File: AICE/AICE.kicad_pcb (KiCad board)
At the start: 2 copper layers, 90 x 85 mm, 140 parts, among them J1 Conn_02x10_Odd_Even, J2 Conn_02x10_Odd_Even, J3 Conn_01x03, J4 USB_A, J5 Conn_02x10_Odd_Even, J6 Conn_02x10_Odd_Even, J8 USB_B_Micro, Q1 S8550, U1 ICE40UP5K-SG48ITR, U11 DVP_PORT, U12 SMS, U13 ZLDO1117G33TA, U14 XC6206P122MR, U15 ZLDO1117G33TA, U16 ZLDO1117G18TA, U17 XC6206P282MR, U18 XC6206P152MR, U2 ASFLMB-24.00MHZ-LC-T, U3 SMS, U4 W25Q, U5 HX711, U6 Omega2+, U7 SMS, U8 SRF2012, U9 M1&M1W

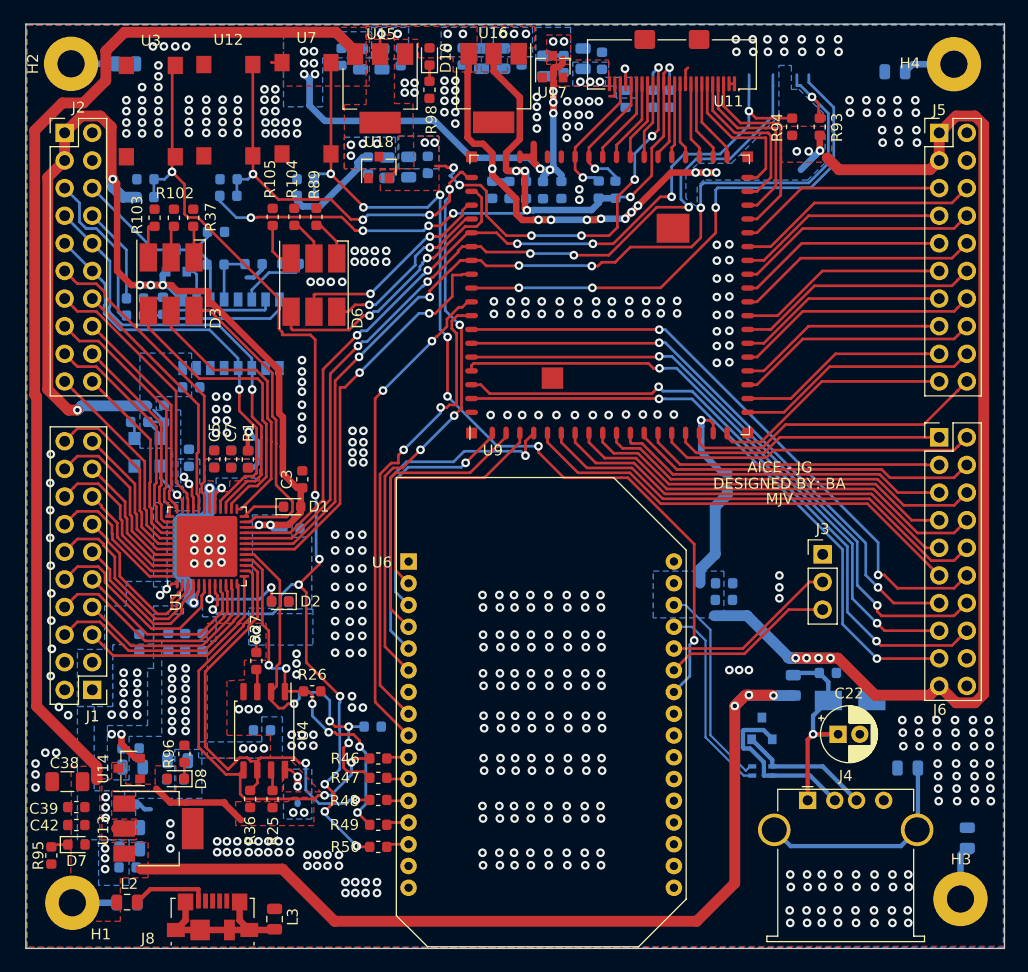
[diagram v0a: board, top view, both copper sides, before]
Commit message: Add files via upload
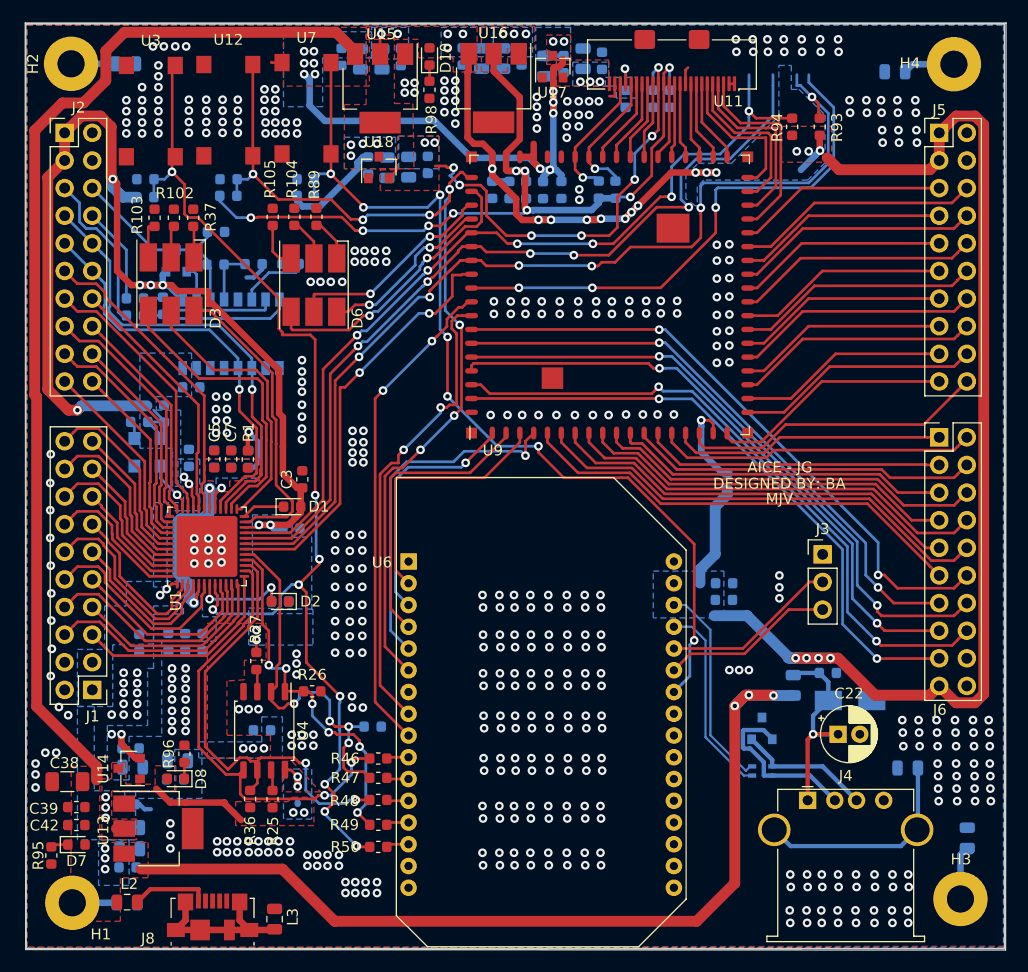
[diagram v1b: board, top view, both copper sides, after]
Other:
- board size 90 x 85 mm -> 90.2 x 85.2 mm
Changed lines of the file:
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@@
   (general
     (thickness 1.6)
-    (drawings 10)
+    (drawings 14)
     (tracks 2330)
     (zones 0)
@@
     )
   )
+  (gr_line (start 123.15 63.9) (end 123.1 149.15) (layer Edge.Cuts) (width 0.1))
+  (gr_line (start 32.95 63.9) (end 123.15 63.9) (layer Edge.Cuts) (width 0.1))
+  (gr_line (start 33 149.1) (end 32.95 63.9) (layer Edge.Cuts) (width 0.1))
+  (gr_line (start 123.1 149.15) (end 33 149.1) (layer Edge.Cuts) (width 0.1))
+  (gr_line (start 123 148.998) (end 33.006 148.998) (layer Edge.Cuts) (width 0.05))
+  (gr_line (start 33.006 148.998) (end 33.006 63.998) (layer Edge.Cuts) (width 0.05))
+  (gr_line (start 33.006 63.998) (end 123 63.998) (layer Edge.Cuts) (width 0.05))
+  (gr_line (start 123 63.998) (end 123 143) (layer Edge.Cuts) (width 0.05))
   (gr_text MJV (at 102.3 107.65) (layer F.SilkS)
     (effects (font (size 1 1) (thickness 0.25)))
@@
     (effects (font (size 1 1) (thickness 0.15) italic))
   )
-  (gr_line (start 123 148.998) (end 33.006 148.998) (layer Edge.Cuts) (width 0.05))
   (gr_line (start 123 143) (end 123 149) (layer Edge.Cuts) (width 0.05))
-  (gr_line (start 123 63.998) (end 123 143) (layer Edge.Cuts) (width 0.05))
-  (gr_line (start 33.006 63.998) (end 123 63.998) (layer Edge.Cuts) (width 0.05))
-  (gr_line (start 33.006 148.998) (end 33.006 63.998) (layer Edge.Cuts) (width 0.05))
   (via (at 47.75 66.05) (size 0.8) (drill 0.4) (layers F.Cu B.Cu) (net 0))
   (via (at 45.7 66.05) (size 0.8) (drill 0.4) (layers F.Cu B.Cu) (net 0))
